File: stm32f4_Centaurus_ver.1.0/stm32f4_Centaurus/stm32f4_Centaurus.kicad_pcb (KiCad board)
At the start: 2 copper layers, 100 x 79 mm, 211 parts, among them IC1 PIC24FJ64GB004, P1 PICKit3, P10 XA2_12V, P11 CAN0, P12 CAN1, P13 CAN0, P14 CAN1, P15 SERIAL2, P16 SERIAL0, P17 XA2_5V, P18 SWD, P2 SERIAL5_SBDBT, P23 A/D, P24 PWM, P25 A/D_batt, P26 PWM_batt, P27 EMERGENCY_CHECK, P28 I/O_3.3V, P29 I/O_5V, P3 ENC0, P30 I/O_3.3V_batt, P31 I/O_5V_batt, P4 ENC2, P5 SERIAL1, P6 ENC3, P7 ENC1, P8 SERIAL4, P9 SERIAL3, Q1 FET_P, Q2 FET_P, Q3 FET_P, Q4 NPN, Q5 NPN, Q6 FET_P, Q7 FET_N, SW1 Main_POWER, SW2 SW1, SW3 SW0, SW4 SW2, SW5 SW3, U1 STM32F407VG, U10 LOGO, U12 25LC010A, U13 LOGO, U2 AZ1086H, U3 MCP2221A, U4 AP3211, U5 MAX3051, U6 MAX3051, U7 AQM1602_BL, U8 OSTBABS4C2B, U9 LOGO, X1 8MHz

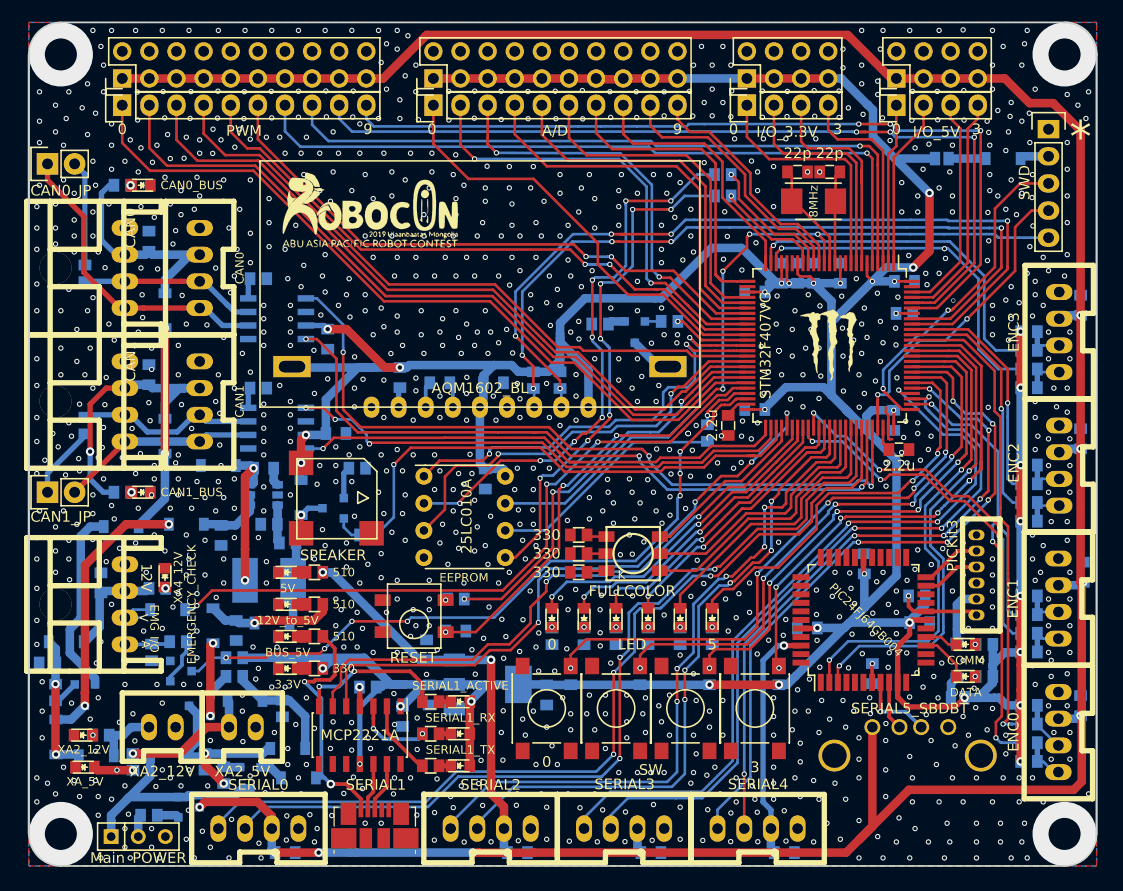
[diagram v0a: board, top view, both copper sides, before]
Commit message: とりあえず、問題なければ完了.
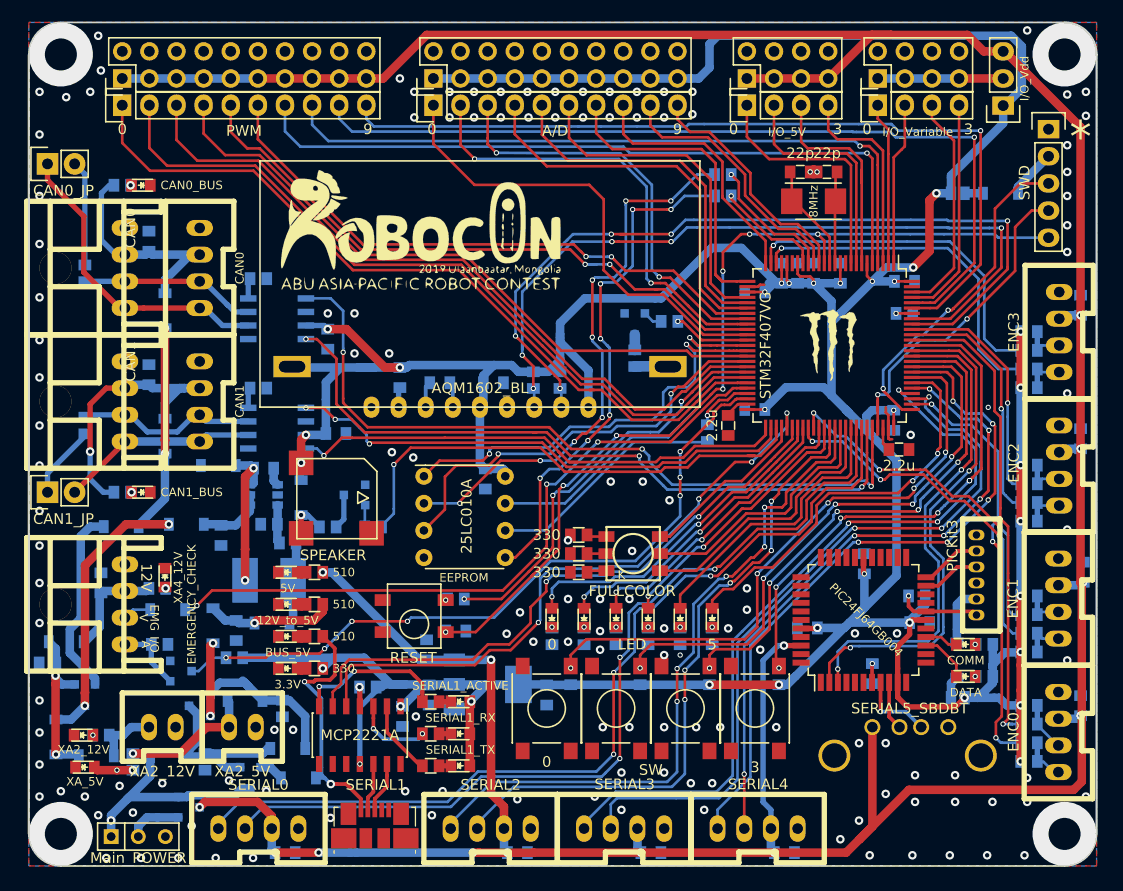
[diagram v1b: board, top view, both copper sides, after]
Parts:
- removed R27, R29, R31, R32, R70: 10, Mizz_lib:R_0603
- added JP5: I/O_Vdd, Mizz_lib:Pin_Header_Straight_1x03, F.Cu at (144.2, 66.8)
- P28: value I/O_3.3V -> I/O_5V
- P29: value I/O_5V -> I/O_Variable
- P30: value I/O_3.3V_batt -> I/O_5V_batt
- P31: value I/O_5V_batt -> I/O_Variable
- U13: footprint Mizz_lib:Robocon2019_18.8x18.8_silk -> Mizz_lib:Robocon2019_30.0x30.0_silk
- moved R53 6.15 mm to (81.0, 106.2)
- moved U13 5.15 mm to (89.8, 78.8)
- moved R43 4.56 mm to (109.8, 90.5), turned to 90 degrees
- moved JP3 3.58 mm to (140.0, 75.0)
- moved D40 3.26 mm to (144.0, 75.0)
- moved Q4 2.36 mm to (83.5, 103.2)
- moved P29 1.75 mm to (132.5, 66.8)
- moved P31 1.75 mm to (132.5, 64.2)
- moved R71 1.06 mm to (65.2, 117.2), turned to 0 degrees
- moved U10 0.96 mm to (69.8, 73.2)
- moved R51 0.90 mm to (85.2, 106.2)
- moved Q5 0.75 mm to (109.8, 87.2)
- moved C11 0.25 mm to (125.2, 73.0)
- moved C13 0.25 mm to (127.8, 73.0)
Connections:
- IC1 pad 2: /USART2_TX -> /USART2_RX
- IC1 pad 3: /USART2_RX -> /USART2_TX
- P30 pad 1: +3.3V -> +5V
- P30 pad 3: +3.3V -> +5V
- P30 pad 5: +3.3V -> +5V
- P30 pad 7: +3.3V -> +5V
- P31 pad 1: +5V -> Net-(JP5-Pad2)
- P31 pad 3: +5V -> Net-(JP5-Pad2)
- P31 pad 5: +5V -> Net-(JP5-Pad2)
- P31 pad 7: +5V -> Net-(JP5-Pad2)
- Q1 pad 1: Net-(Q1-Pad1) -> /XA_12V
- Q2 pad 1: Net-(Q2-Pad1) -> Net-(D11-Pad2)
- Q3 pad 1: Net-(Q3-Pad1) -> Net-(D27-Pad1)
- Q4 pad 2: Net-(Q4-Pad2) -> GND
- Q4 pad 3: Net-(D20-Pad1) -> Net-(Q4-Pad3)
- Q7 pad 1: Net-(Q7-Pad1) -> Net-(P27-Pad4)
- R53 pad 1: Net-(Q4-Pad2) -> Net-(D20-Pad1)
- R53 pad 2: GND -> Net-(Q4-Pad3)
- SW1 pad 2: Net-(R32-Pad2) -> Net-(Q6-Pad1)
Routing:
- net +3.3V: track 431.1 -> 447.5 mm
- net +5V: track 329.5 -> 344.9 mm
- net Net-(JP5-Pad2): track 0.00 -> 11.8 mm
- net Net-(R43-Pad1): track 0.00 -> 4.49 mm
- net Net-(Q7-Pad1): track 4.32 -> 0.00 mm
- net Net-(D11-Pad2): track 10.7 -> 14.7 mm
- net Net-(Q4-Pad3): track 0.00 -> 3.30 mm
- net Net-(Q5-Pad3): track 4.54 -> 1.42 mm
- net Net-(Q6-Pad1): track 2.05 -> 5.07 mm
- net Net-(Q4-Pad2): track 2.99 -> 0.00 mm
- net /ADC12_IN9: track 41.6 -> 44.3 mm
- net Net-(Q1-Pad1): track 2.43 -> 0.00 mm
- net Net-(Q2-Pad1): track 2.41 -> 0.00 mm
- net Net-(P27-Pad4): track 4.29 -> 6.66 mm
- net /XA_12V: track 12.5 -> 14.8 mm
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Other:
- board text added: "Desgined by A.Mizuta in 2019/04/02."
- board text added: "STM32F407VGT6 Board "Centaurus" ver.1.1."
- board text removed: "Desgined by A.Mizuta in 2019/02/08."
- board text removed: "STM32F407VGT6 Board "Centaurus" ver.1.0."
